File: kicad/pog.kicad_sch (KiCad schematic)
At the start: 179 parts, among them J1 USB_C_Receptacle, U1 ATmega32U4-A

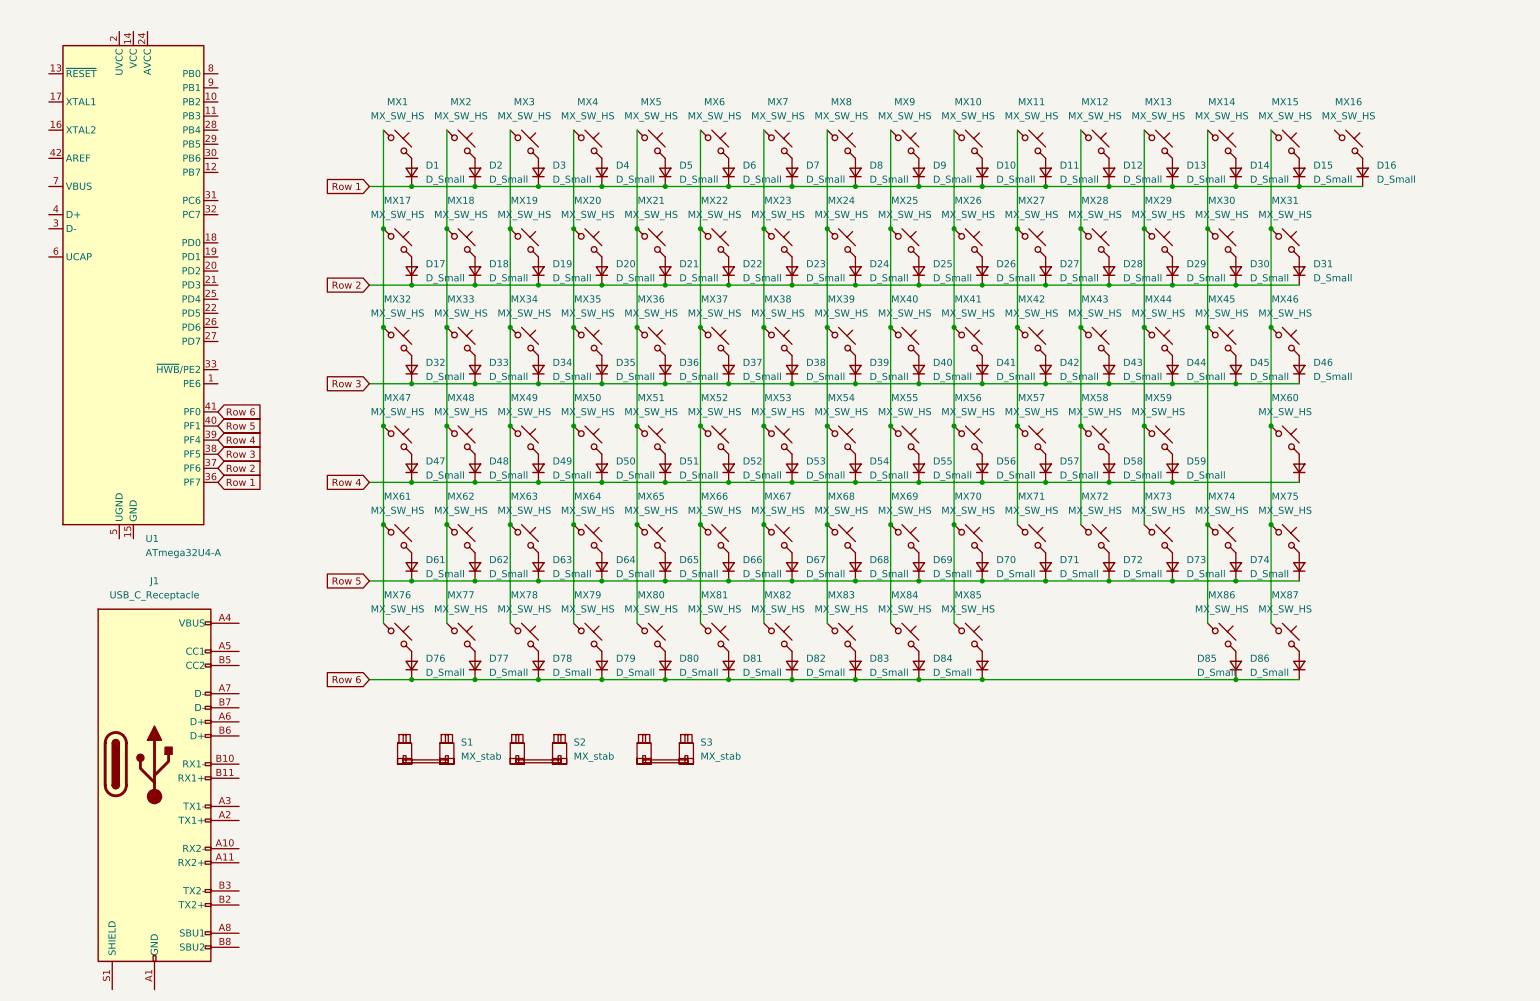
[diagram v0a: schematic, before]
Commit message: schematic done
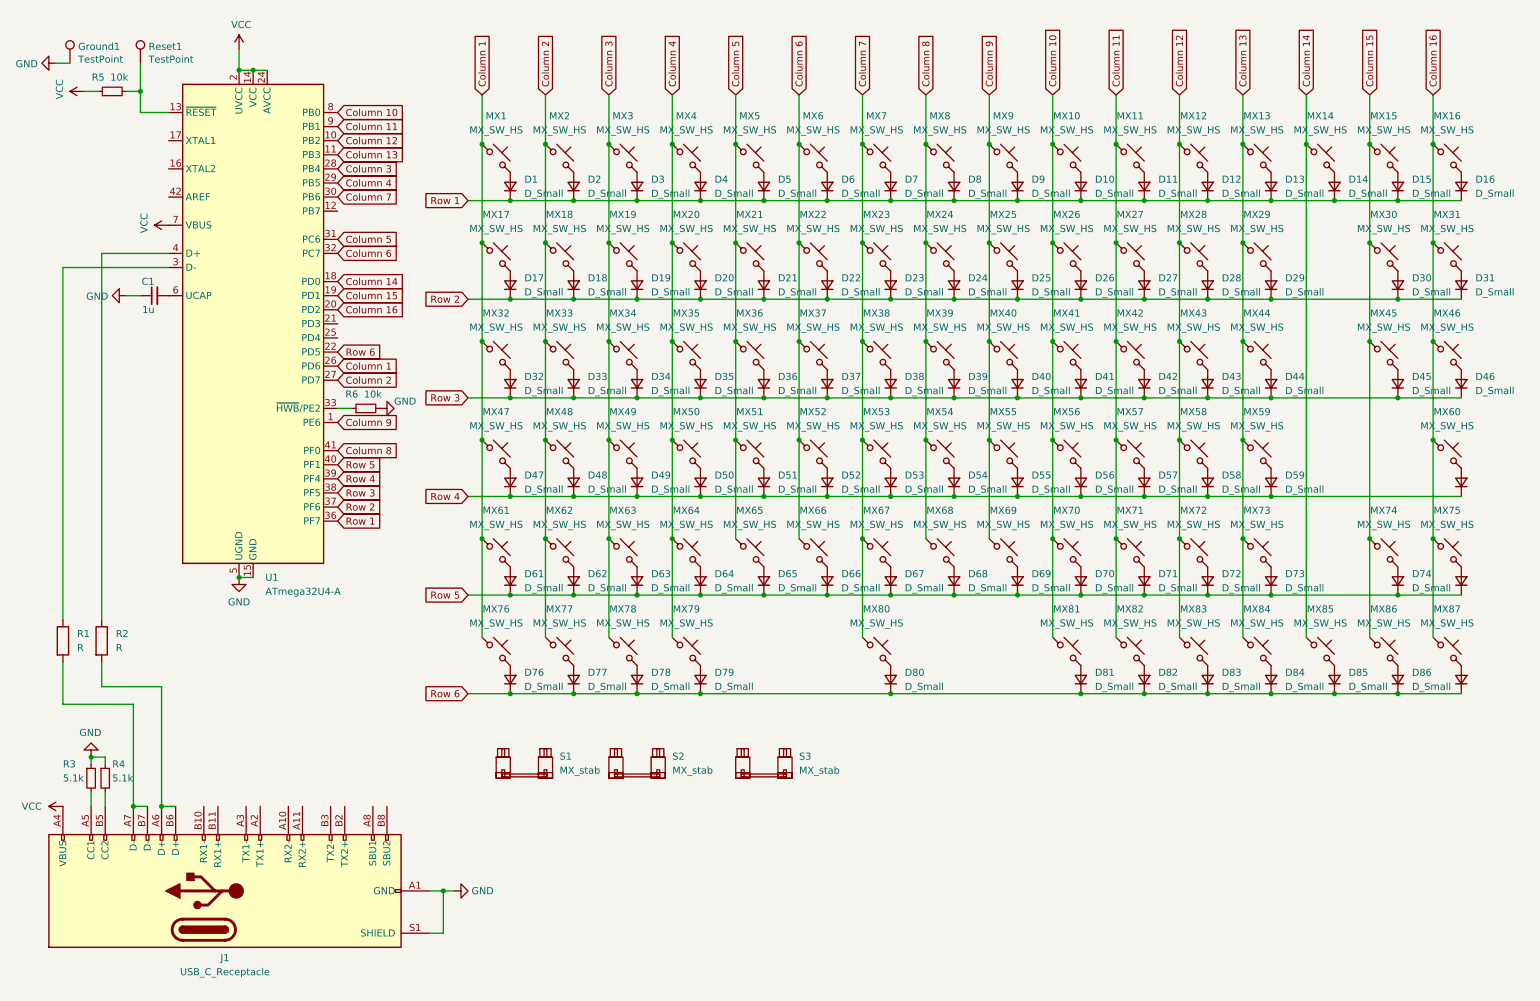
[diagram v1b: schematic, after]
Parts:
- added C1: 1u, Capacitor_SMD:C_1206_3216Metric, symbol Device:C_Small
- added Ground1, Reset1: TestPoint, TestPoint:TestPoint_THTPad_2.0x2.0mm_Drill1.0mm, symbol Connector:TestPoint
- added R1, R2: R, Resistor_SMD:R_1206_3216Metric, symbol Device:R
- added R3, R4: 5.1k, Resistor_SMD:R_1206_3216Metric, symbol Device:R_Small
- added R5, R6: 10k, Resistor_SMD:R_1206_3216Metric, symbol Device:R_Small
- J1: footprint (none) -> USB_C:USB_C_Receptacle_HRO_TYPE-C-31-M-12
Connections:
- net Row 6: now also U1.22 (PD5); no longer U1.41 (PF0)
- net Column 3: now reaches MX19.1, MX3.1, MX34.1, MX49.1, MX63.1, MX78.1
- net Column 3: now also U1.28 (PB4)
- net Column 6: now reaches MX22.1, MX37.1, MX52.1, MX6.1, MX66.1
- net Column 6: now also U1.32 (PC7); no longer MX81.1
- net Column 2: now reaches MX18.1, MX2.1, MX33.1, MX48.1, MX62.1, MX77.1
- net Column 2: now also U1.27 (PD7)
- net Column 16: now reaches MX31.1, MX46.1, MX60.1, MX75.1, MX87.1
- net Column 16: now also MX16.1, U1.20 (PD2); no longer MX15.1
- net Column 15: now reaches MX30.1, MX45.1, MX74.1, MX86.1
- net Column 15: now also MX15.1, U1.19 (PD1); no longer MX14.1
- net Column 12: now reaches MX12.1, MX28.1, MX43.1, MX58.1, MX72.1
- net Column 12: now also MX83.1, U1.10 (PB2)
- net Column 10: now reaches MX10.1, MX26.1, MX41.1, MX56.1, MX70.1
- net Column 10: now also MX81.1, U1.8 (PB0); no longer MX85.1
- net Column 7: now reaches MX23.1, MX38.1, MX53.1, MX67.1, MX7.1
- net Column 7: now also MX80.1, U1.30 (PB6); no longer MX82.1
- net Column 9: now reaches MX25.1, MX40.1, MX55.1, MX69.1, MX9.1
- net Column 9: now also U1.1 (PE6); no longer MX84.1
- net Column 8: now reaches MX24.1, MX39.1, MX54.1, MX68.1, MX8.1
- net Column 8: now also U1.41 (PF0); no longer MX83.1
- net Column 4: now reaches MX20.1, MX35.1, MX4.1, MX50.1, MX64.1, MX79.1
- net Column 4: now also U1.29 (PB5)
- net Column 5: now reaches MX21.1, MX36.1, MX5.1, MX51.1, MX65.1
- net Column 5: now also U1.31 (PC6); no longer MX80.1
- net Column 1: now reaches MX1.1, MX17.1, MX32.1, MX47.1, MX61.1, MX76.1
- net Column 1: now also U1.26 (PD6)
- net Column 13: now reaches MX13.1, MX29.1, MX44.1, MX59.1, MX73.1
- net Column 13: now also MX84.1, U1.11 (PB3)
- net Column 11: now reaches MX11.1, MX27.1, MX42.1, MX57.1, MX71.1
- net Column 11: now also MX82.1, U1.9 (PB1)
- net at U1.13 (~{RESET}): now also R5.2, Reset1.1
- net VCC: now reaches U1.14 (VCC), U1.34 (VCC)
- net VCC: now also J1.A4 (VBUS), J1.A9 (VBUS), J1.B4 (VBUS), J1.B9 (VBUS), U1.2 (UVCC), U1.24 (AVCC), U1.44 (AVCC), U1.7 (VBUS), R5.1
- net GND: now reaches U1.15 (GND), U1.23 (GND), U1.35 (GND), U1.43 (GND)
- net GND: now also J1.A1 (GND), J1.A12 (GND), J1.B1 (GND), J1.B12 (GND), J1.S1 (SHIELD), U1.5 (UGND), C1.1, Ground1.1, R3.1, R4.1, R6.2
- net Column 14: now reaches U1.18 (PD0)
- net Column 14: now also MX14.1, MX85.1
- net at U1.3 (D-): now also R1.1
- net at U1.33 (~{HWB}/PE2): now also R6.1
- net at U1.4 (D+): now also R2.1
- net at U1.6 (UCAP): now also C1.2
- net at J1.A5 (CC1): now also R3.2
- net at J1.A6 (D+): now also J1.B6 (D+), R2.2
- net at J1.A7 (D-): now also J1.B7 (D-), R1.2
- net at J1.B5 (CC2): now also R4.2
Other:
- moved on the sheet: D1, D10, D11, D12, D13, D14, D15, D16, D17, D18, D19, D2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

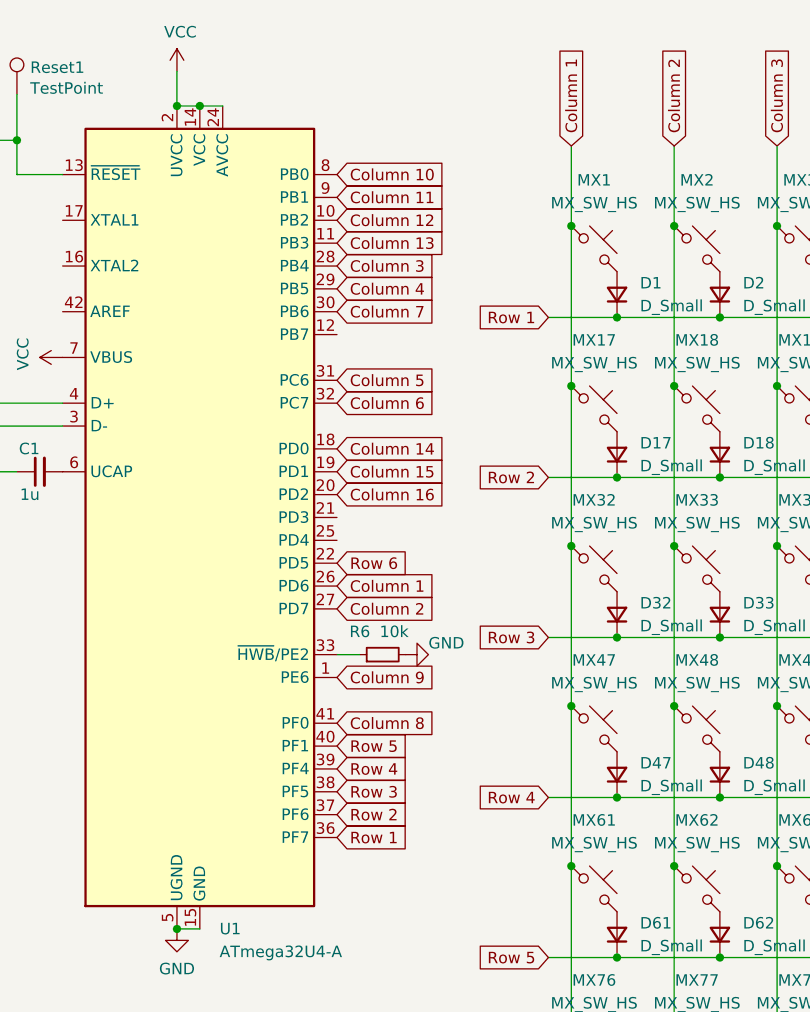
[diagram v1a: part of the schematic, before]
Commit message: complete basic pcb design
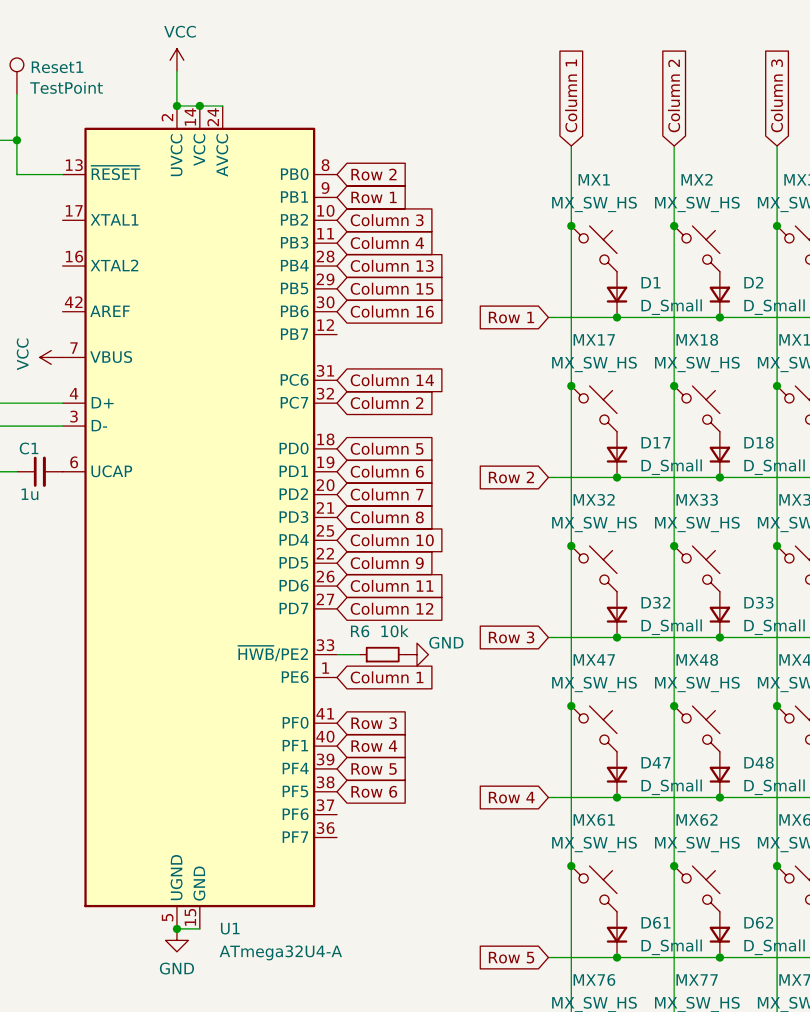
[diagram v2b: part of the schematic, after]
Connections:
- net Column 1: now also U1.1 (PE6); no longer U1.26 (PD6)
- net Column 10: now also U1.25 (PD4); no longer U1.8 (PB0)
- net Column 11: now also U1.26 (PD6); no longer U1.9 (PB1)
- net Column 12: now also U1.27 (PD7); no longer U1.10 (PB2)
- net Column 13: now also U1.28 (PB4); no longer U1.11 (PB3)
- net Column 14: now also U1.31 (PC6); no longer U1.18 (PD0)
- net Column 15: now also U1.29 (PB5); no longer U1.19 (PD1)
- net Column 16: now also U1.30 (PB6); no longer U1.20 (PD2)
- net Column 2: now also U1.32 (PC7); no longer U1.27 (PD7)
- net Column 3: now also U1.10 (PB2); no longer U1.28 (PB4)
- net Column 4: now also U1.11 (PB3); no longer U1.29 (PB5)
- net Column 5: now also U1.18 (PD0); no longer U1.31 (PC6)
- net Column 6: now also U1.19 (PD1); no longer U1.32 (PC7)
- net Column 7: now also U1.20 (PD2); no longer U1.30 (PB6)
- net Column 8: now also U1.21 (PD3); no longer U1.41 (PF0)
- net Column 9: now also U1.22 (PD5); no longer U1.1 (PE6)
- net Row 1: now also U1.9 (PB1); no longer U1.36 (PF7)
- net Row 2: now also U1.8 (PB0); no longer U1.37 (PF6)
- net Row 3: now also U1.41 (PF0); no longer U1.38 (PF5)
- net Row 4: now also U1.40 (PF1); no longer U1.39 (PF4)
- net Row 5: now also U1.39 (PF4); no longer U1.40 (PF1)
- net Row 6: now also U1.38 (PF5); no longer U1.22 (PD5)
